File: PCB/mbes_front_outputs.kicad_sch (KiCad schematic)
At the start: 55 parts, among them IC2 BDX34C, IC3 BDX34C, Q1 D45VH10, Q10 BC337, Q14 D45VH10, Q15 D45VH10, Q2 D45VH10, Q3 BC337, Q4 BC337, Q5 BC337, Q6 BC337, Q7 BC337, Q8 BC337, Q9 BC337

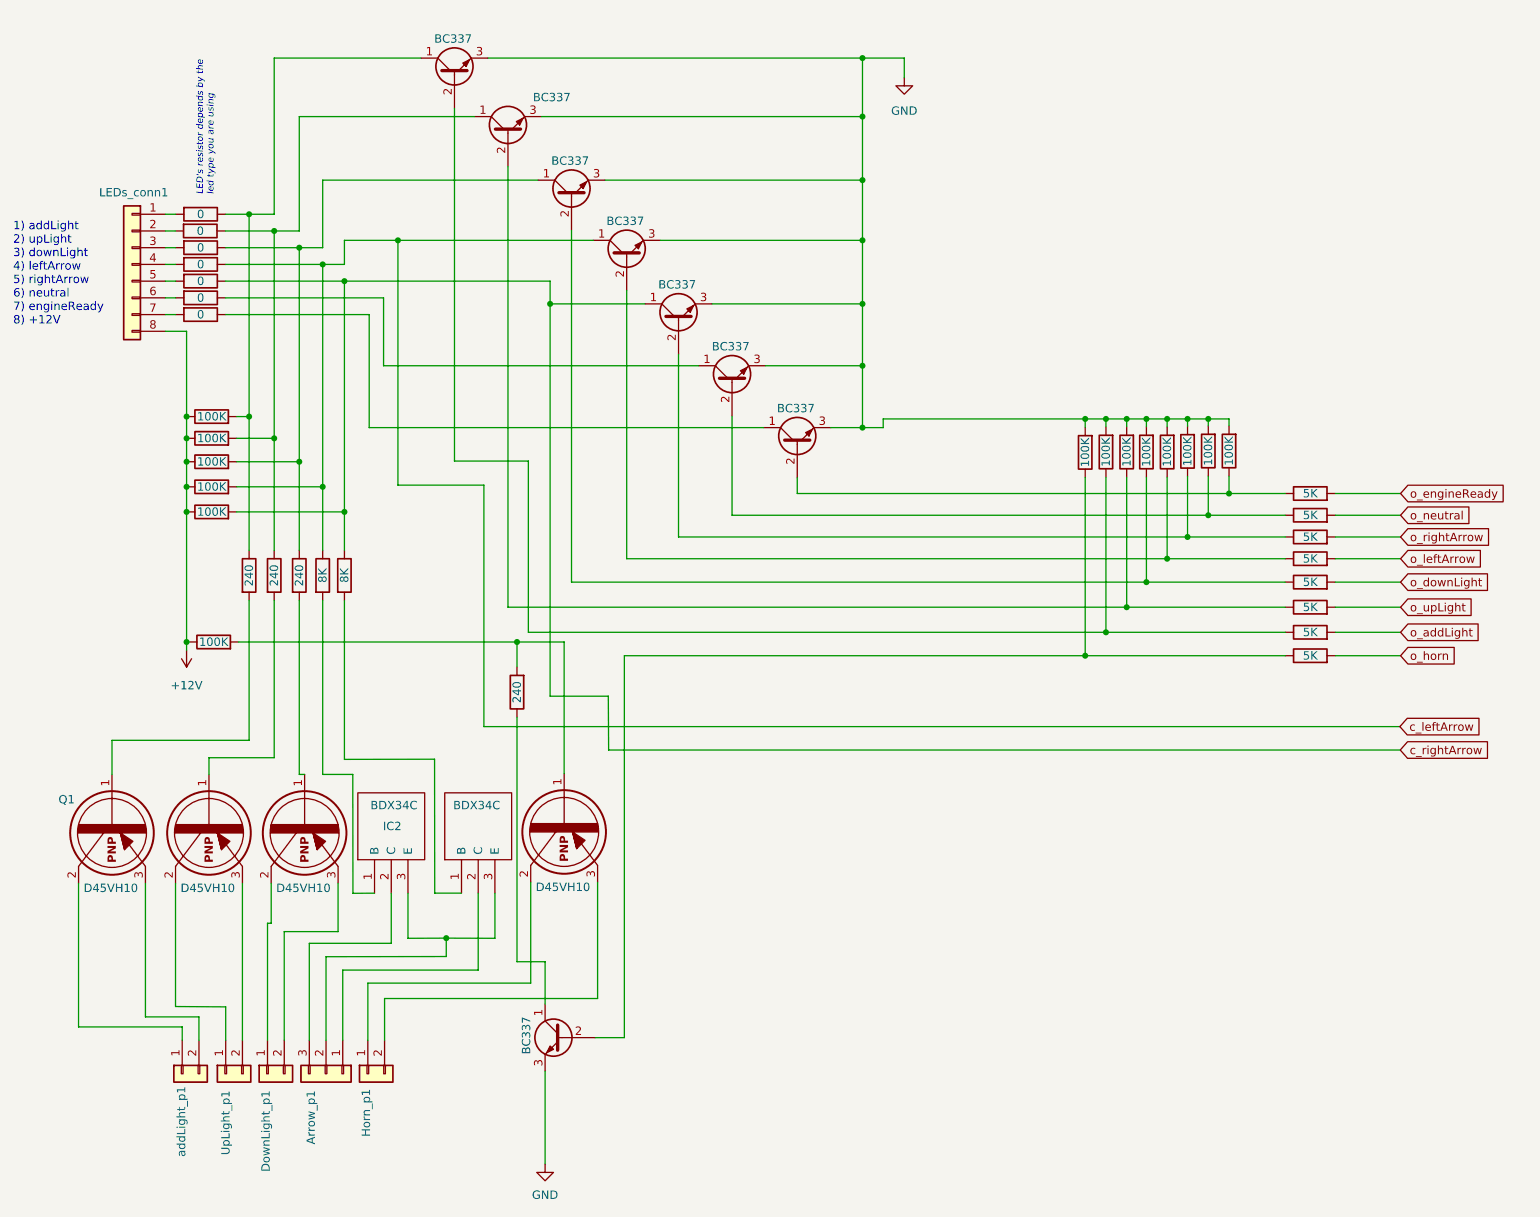
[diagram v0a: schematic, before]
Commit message: Merged files
These files have been merged by remotes/origin/ATmega16__dualPCB__bluetoothCockpit branch
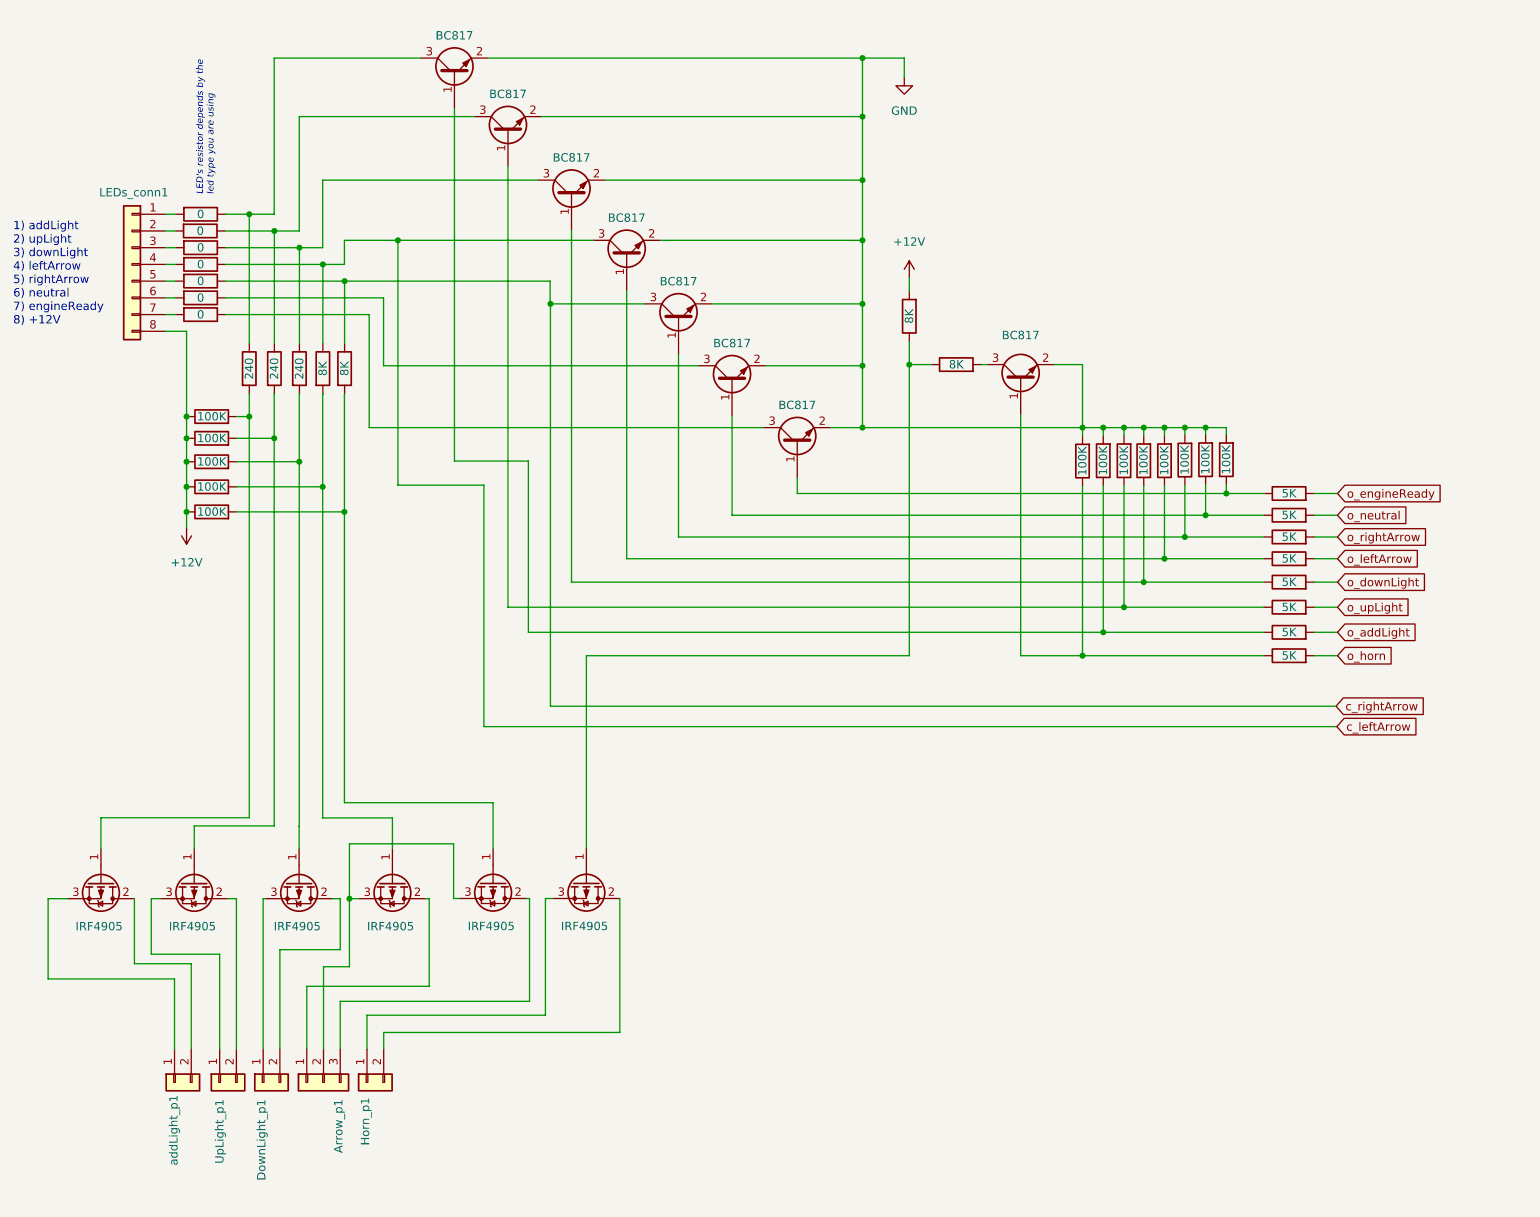
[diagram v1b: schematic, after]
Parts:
- removed IC2, IC3: BDX34C, BDX34C:TO270P460X1020X2008-3P, symbol BDX34C:BDX34C
- removed Q1, Q14, Q15, Q2: D45VH10, Package_TO_SOT_THT:TO-220-3_Vertical, symbol D45VH10:D45VH10
- removed Q10, Q3, Q4, Q5, Q6, Q7, Q8, Q9: BC337, Package_TO_SOT_THT:TO-92L_Inline_Wide, symbol Transistor_BJT:BC337
- added Q1, Q14, Q15, Q19, Q2, Q20, Q21, Q3: BC817, Package_TO_SOT_SMD:SOT-23, symbol Transistor_BJT:BC817
- added Q4, Q5, Q6, Q7, Q8, Q9: IRF4905, Package_TO_SOT_THT:TO-220-3_Vertical, symbol Transistor_FET:IRF4905
- RA1, RA2, RA3, RA4, RA5, RA6, RA9: footprint Resistor_THT:R_Axial_DIN0207_L6.3mm_D2.5mm_P10.16mm_Horizontal -> Resistor_SMD:R_1206_3216Metric
- RA10, RA11, RA12: footprint Resistor_THT:R_Axial_DIN0414_L11.9mm_D4.5mm_P15.24mm_Horizontal -> Resistor_SMD:R_1206_3216Metric
- RA13, RA14, RA16, RA17, RA18, RA19, RA20, RA21, RA22, RA24, RA25, RA26, RA27, RA28, RA32, RA34, RA35, RA36, RA37, RA38, RA39, RA40, RA7: footprint Resistor_THT:R_Axial_DIN0207_L6.3mm_D2.5mm_P7.62mm_Horizontal -> Resistor_SMD:R_1206_3216Metric
- RA15: value 240 -> 8K; footprint Resistor_THT:R_Axial_DIN0414_L11.9mm_D4.5mm_P15.24mm_Horizontal -> Resistor_SMD:R_1206_3216Metric
- RA42: value 100K -> 8K; footprint Resistor_THT:R_Axial_DIN0207_L6.3mm_D2.5mm_P7.62mm_Horizontal -> Resistor_SMD:R_1206_3216Metric
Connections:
- net +12V: now also RA42.2; no longer RA42.1
- net GND: now also Q1.2 (E), Q14.2 (E), Q15.2 (E), Q19.2 (E), Q2.2 (E), Q20.2 (E), Q21.2 (E), Q3.2 (E)
- net c_leftArrow: now also Q15.3 (C); no longer RA27.2
- net c_rightArrow: now also Q19.3 (C); no longer RA28.2
- net at RA15.1: now also RA42.1, Q9.1 (G)
- net at RA15.2: now also Q3.3 (C); no longer RA42.2
- net at RA1.1, RA10.1: now also Q1.3 (C); no longer RA24.2
- net at RA32.1, RA7.1: now also Q3.1 (B)
- net at RA10.2: now also RA24.2, Q4.1 (G)
- net at addLight_p1.1 (Pin_1): now also Q4.3 (S)
- net at addLight_p1.2 (Pin_2): now also Q4.2 (D)
- net at RA12.1, RA3.1: now also Q14.3 (C); no longer RA26.2
- net at RA6.1: now also Q20.3 (C)
- net at RA17.1, RA39.1: now also Q20.1 (B)
- net at RA20.1, RA36.1: now also Q14.1 (B)
- net at RA13.2: now also RA27.2, Q7.1 (G)
- net at RA22.1, RA34.1: now also Q1.1 (B)
- net at RA19.1, RA37.1: now also Q15.1 (B)
- net at RA11.1, RA2.1: now also Q2.3 (C); no longer RA25.2
- net at RA21.1, RA35.1: now also Q2.1 (B)
- net at DownLight_p1.1 (Pin_1): now also Q6.3 (S)
- net at DownLight_p1.2 (Pin_2): now also Q6.2 (D)
- net at Horn_p1.1 (Pin_1): now also Q9.3 (S)
- net at Horn_p1.2 (Pin_2): now also Q9.2 (D)
- net at RA11.2: now also RA25.2, Q5.1 (G)
- net at UpLight_p1.1 (Pin_1): now also Q5.3 (S)
- net at UpLight_p1.2 (Pin_2): now also Q5.2 (D)
- net at RA14.2: now also RA28.2, Q8.1 (G)
- net at Arrow_p1.3 (Pin_3): now also Q8.2 (D)
- net at Arrow_p1.2 (Pin_2): now also Q7.3 (S), Q8.3 (S)
- net at RA18.1, RA38.1: now also Q19.1 (B)
- net at RA9.1: now also Q21.3 (C)
- net at RA16.1, RA40.1: now also Q21.1 (B)
- net at Arrow_p1.1 (Pin_1): now also Q7.2 (D)
- net at RA12.2: now also RA26.2, Q6.1 (G)
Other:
- moved on the sheet: Arrow_p1, DownLight_p1, Horn_p1, UpLight_p1, addLight_p1
